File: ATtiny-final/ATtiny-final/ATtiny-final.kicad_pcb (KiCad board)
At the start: 2 copper layers, 19.5 x 19.4 mm, 8 parts, among them J1 Conn_01x07_Male, J2 Conn_01x07_Male, U1 ATtiny424-X

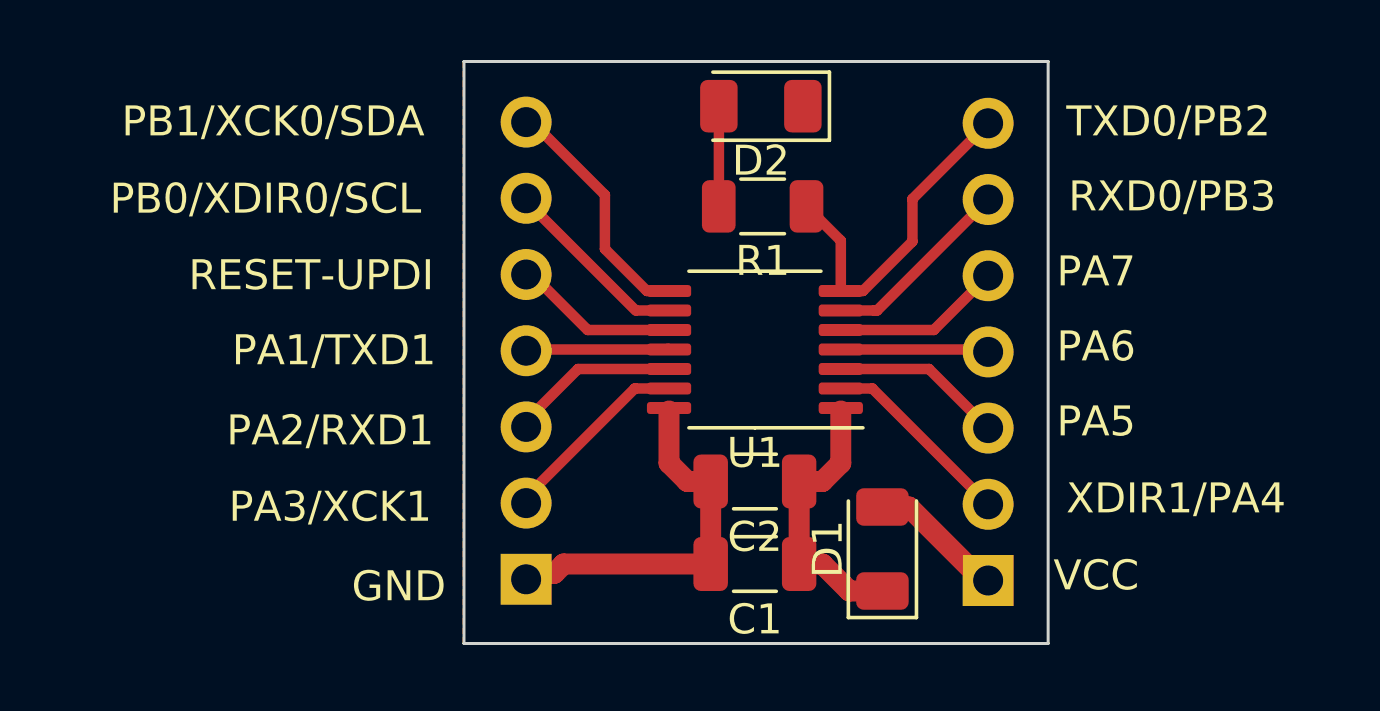
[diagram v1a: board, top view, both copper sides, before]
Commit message: platinen angepasst
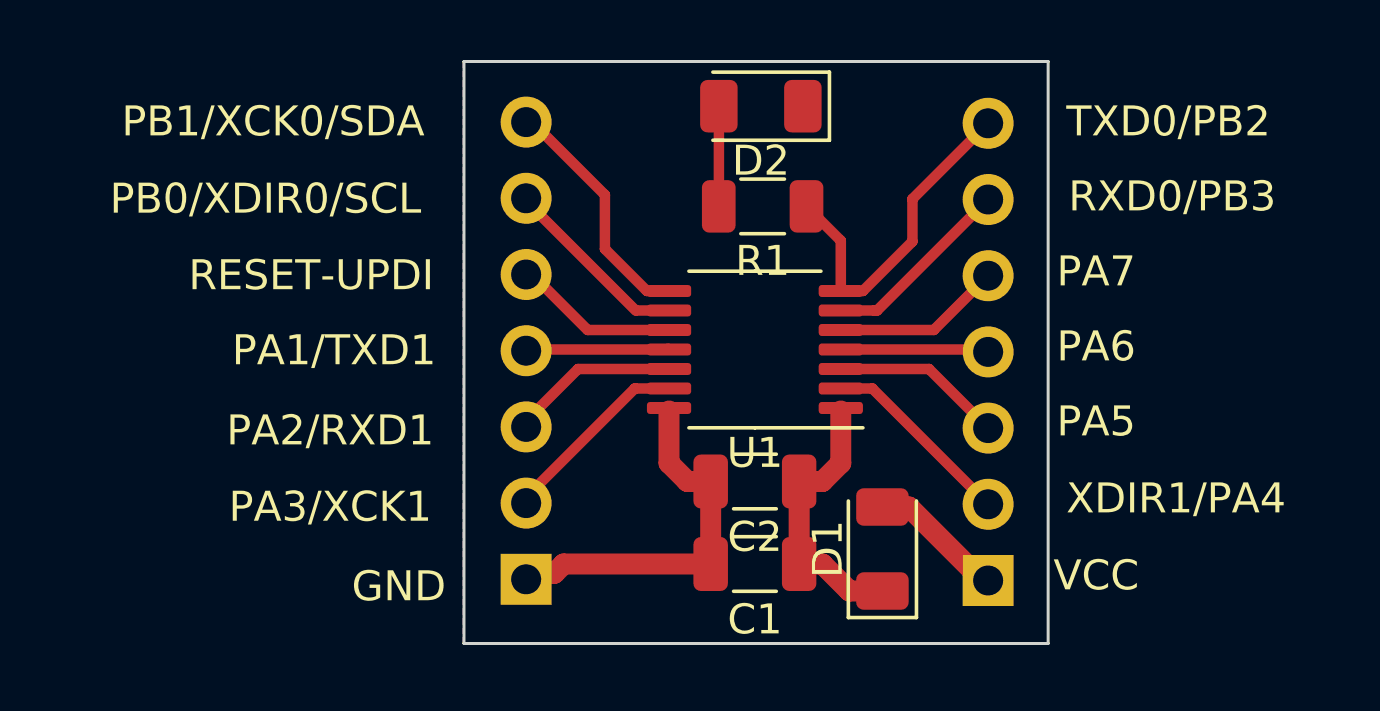
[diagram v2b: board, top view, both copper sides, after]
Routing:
- added copper zone on B.Cu, net GND
- added copper zone on In1.Cu, net GND
- added copper zone on In2.Cu, net GND
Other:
- copper layers 2 -> 4
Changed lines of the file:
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@@
   (layers
     (0 "F.Cu" signal)
+    (1 "In1.Cu" signal)
+    (2 "In2.Cu" signal)
     (31 "B.Cu" signal)
     (32 "B.Adhes" user "B.Adhesive")
@@
       (layer "F.Mask" (type "Top Solder Mask") (thickness 0.01))
       (layer "F.Cu" (type "copper") (thickness 0.035))
-      (layer "dielectric 1" (type "core") (thickness 1.51) (material "FR4") (epsilon_r 4.5) (loss_tangent 0.02))
+      (layer "dielectric 1" (type "prepreg") (thickness 0.1) (material "FR4") (epsilon_r 4.5) (loss_tangent 0.02))
+      (layer "In1.Cu" (type "copper") (thickness 0.035))
+      (layer "dielectric 2" (type "core") (thickness 1.24) (material "FR4") (epsilon_r 4.5) (loss_tangent 0.02))
+      (layer "In2.Cu" (type "copper") (thickness 0.035))
+      (layer "dielectric 3" (type "prepreg") (thickness 0.1) (material "FR4") (epsilon_r 4.5) (loss_tangent 0.02))
       (layer "B.Cu" (type "copper") (thickness 0.035))
       (layer "B.Mask" (type "Bottom Solder Mask") (thickness 0.01))
@@
     (pad_to_mask_clearance 0)
     (pcbplotparams
-      (layerselection 0x0001000_7fffffff)
+      (layerselection 0x0001000_ffffffff)
       (plot_on_all_layers_selection 0x0000000_00000000)
       (disableapertmacros false)
@@
     (connect_pads (clearance 0.5))
     (min_thickness 0.25) (filled_areas_thickness no)
+    (fill yes (thermal_gap 0.5) (thermal_bridge_width 0.5))
+    (polygon
+      (pts
+        (xy 141.5 89.4)
+        (xy 161 89.4)
+        (xy 161 108.8)
+        (xy 141.5 108.8)
+      )
+    )
+  )
+  (zone (net 1) (net_name "GND") (layers "In1.Cu" "In2.Cu" "B.Cu") (hatch edge 0.5)
+    (priority 1)
+    (connect_pads (clearance 0.5))
+    (min_thickness 0.25) (filled_areas_thickness no)
